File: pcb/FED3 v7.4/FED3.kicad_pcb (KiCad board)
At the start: 4 copper layers, 108 x 50 mm, 89 parts, among them IC1 MC74VHC1GT125, IC2 TB6612FNG, IC4 RTC PCF8523T, J1 Conn_02x03_Odd_Even, Q2 DMP2035U-7, SW1 Sw, SW2 SPST_TACT-KMR2, U1 ATSAMD21G18A, U2 MIC5504-3.3, U3 MCP73831T, X1 ClockXtal, X2 uXtal, X4 microsd, X5 JST-XH-02

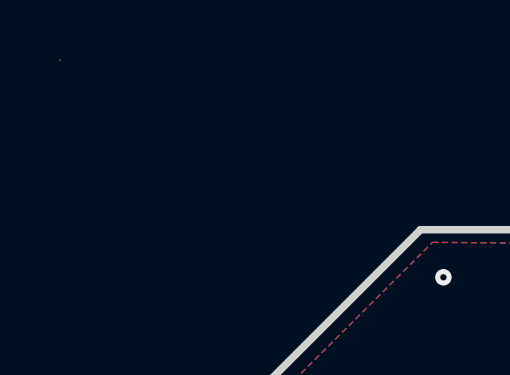
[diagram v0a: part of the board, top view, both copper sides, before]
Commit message: 'ultima versão revista; não em tunning com a versão oficial /Kravitz/FED3
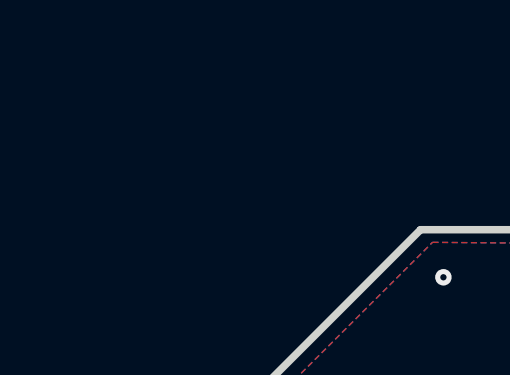
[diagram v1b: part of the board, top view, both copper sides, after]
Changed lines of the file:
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@@
 		(sheetname "/Controller Stage/")
 		(sheetfile "controler stage.kicad_sch")
+		(attr smd)
 		(fp_circle
 			(center 0 0)
@@
 		(sheetname "/IOs Interface/")
 		(sheetfile "IOs Interface.kicad_sch")
+		(attr smd)
 		(fp_line
 			(start -1.45 0.8)
@@
 			)
 		)
-		(property "MPN" "TB6612FNG,C,8,EL "
+		(property "MPN" "TB6612FNG,C,8,EL"
 			(at 0 0 180)
 			(unlocked yes)
@@
 		(sheetname "/")
 		(sheetfile "FED3.kicad_sch")
+		(attr smd)
 		(fp_line
 			(start 4.128 2.536)
@@
 			)
 		)
-		(property "MPN" "ECS-.327-12.5-17X-C-TR "
+		(property "MPN" "ECS-.327-12.5-17X-C-TR"
 			(at 0 0 270)
 			(unlocked yes)
@@
 		(sheetname "/Controller Stage/")
 		(sheetfile "controler stage.kicad_sch")
+		(attr smd)
 		(fp_line
 			(start -4.1 2)
@@
 			)
 		)
-		(property "Description" "DC DC CONVERTER Boost/Inverter 2output ±40V 1.3A"
+		(property "Description" "BUFFER NON-INVERT 1CH 3-STATE"
 			(at 0 0 90)
 			(unlocked yes)
@@
 		(sheetname "/")
 		(sheetfile "FED3.kicad_sch")
-		(attr through_hole)
+		(attr smd)
 		(fp_line
 			(start -3.75 -2.9)
@@
 		(sheetname "/")
 		(sheetfile "FED3.kicad_sch")
-		(attr through_hole exclude_from_bom)
+		(attr through_hole)
 		(fp_line
 			(start -6.35 -0.635)
@@
 		(sheetname "/IOs Interface/")
 		(sheetfile "IOs Interface.kicad_sch")
-		(attr smd exclude_from_pos_files)
+		(attr smd)
 		(fp_line
 			(start 11 3)
@@
 			)
 		)
-		(property "MPN" "SK6812RGBW-BW"
+		(property "MPN" "XT1511RGBW-BW"
 			(at 0 0 180)
 			(unlocked yes)
@@
 			)
 		)
-		(property "MPN" "SK6812RGBW-BW"
+		(property "MPN" "XT1511RGBW-BW"
 			(at 0 0 270)
 			(unlocked yes)
@@
 			)
 		)
-		(property "MPN" "SSSS811101 "
+		(property "MPN" "SSSS811101"
 			(at 0 0 270)
 			(unlocked yes)
@@
 		(sheetname "/")
 		(sheetfile "FED3.kicad_sch")
+		(attr smd)
 		(fp_line
 			(start -3.4 1.75)
@@
 			)
 		)
-		(property "MPN" "SK6812RGBW-BW"
+		(property "MPN" "XT1511RGBW-BW"
 			(at 0 0 180)
 			(unlocked yes)
@@
 			)
 		)
-		(property "MPN" "SK6812RGBW-BW"
+		(property "MPN" "XT1511RGBW-BW"
 			(at 0 0 270)
 			(unlocked yes)
@@
 			)
 		)
-		(property "MPN" "SK6812RGBW-BW"
+		(property "MPN" "XT1511RGBW-BW"
 			(at 0 0 270)
 			(unlocked yes)
@@
 			)
 		)
-		(property "MPN" "SK6812RGBW-BW"
+		(property "MPN" "XT1511RGBW-BW"
 			(at 0 0 270)
 			(unlocked yes)
@@
 			)
 		)
-		(property "MPN" "SK6812RGBW-BW"
+		(property "MPN" "XT1511RGBW-BW"
 			(at 0 0 270)
 			(unlocked yes)
@@
 			)
 		)
-		(property "MPN" "SK6812RGBW-BW"
+		(property "MPN" "XT1511RGBW-BW"
 			(at 0 0 270)
 			(unlocked yes)
@@
 			)
 		)
-		(property "MPN" "SK6812RGBW-BW"
+		(property "MPN" "XT1511RGBW-BW"
 			(at 0 0 270)
 			(unlocked yes)
@@
 			)
 		)
-		(property "MPN" "SK6812RGBW-BW"
+		(property "MPN" "XT1511RGBW-BW"
 			(at 0 0 270)
 			(unlocked yes)
@@
 		)
 		(layer "F.SilkS")
-	)
-	(gr_arc
-		(start 87.48776 74.351613)
-		(mid 87.487765 74.351635)
-		(end 87.48777 74.351657)
-		(stroke
-			(width 0.01)
-			(type default)
-		)
-		(layer "F.SilkS")
